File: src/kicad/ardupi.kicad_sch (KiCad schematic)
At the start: 58 parts, among them J1 RPI-4B-Header, J10 Conn_01x04, J11 TSW-108-08-L-T-RA, J2 Conn_01x10, J3 Conn_01x05, J4 Conn_01x04, J6 Conn_01x05, J7 Conn_01x06, J8 Conn_01x04, J9 Conn_01x02, U1 CAT24C256, U2 ULN2803ADW, U3 PCA9685PW, U4 ADS1115IRUGR, U5 MPU-9250, U6 BMP280

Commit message: version bump
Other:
- title: (none) -> ArduPi
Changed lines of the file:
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@@
   (paper "A3")
   (title_block
-    (date "15 nov 2012")
+    (title "ArduPi")
+    (date "2022-06-05")
+    (rev "0.1.4")
+    (comment 1 "Author: Muhammad Hefny")
+    (comment 2 "Author: Shaun Lloyd")
   )
   (junction (at 325.12 66.04) (diameter 0) (color 0 0 0 0)

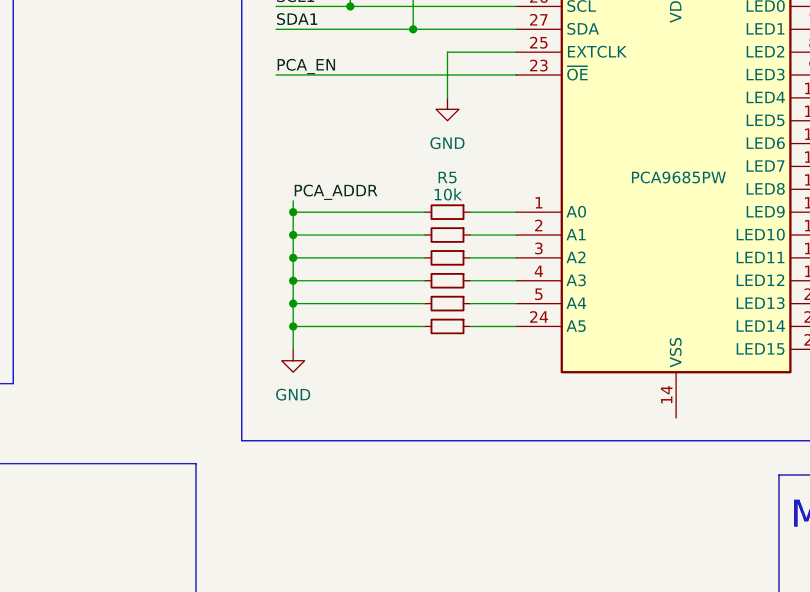
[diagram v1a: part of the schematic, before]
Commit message: elec: PCA9685 jumpers
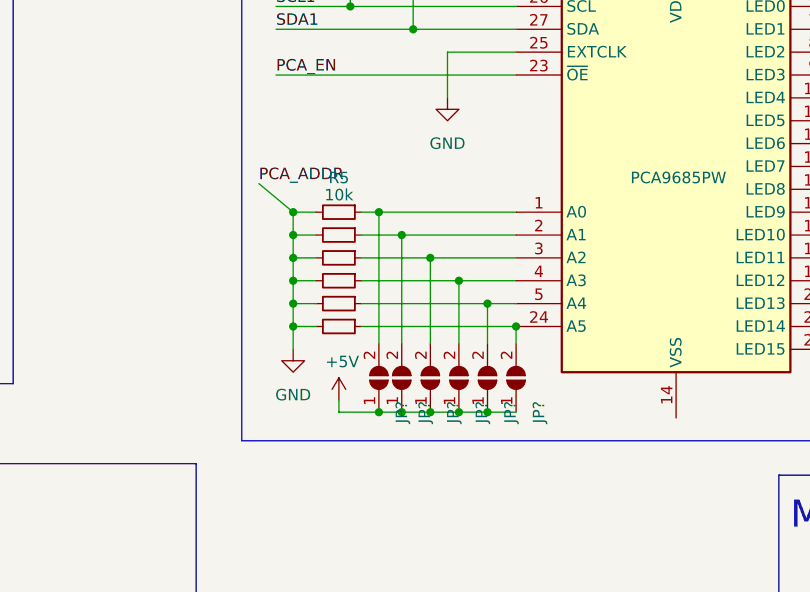
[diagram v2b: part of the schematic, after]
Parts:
- added JP? (x6): ID_WP, symbol Jumper:SolderJumper_2_Open
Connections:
- net +5V: now also JP?.1 (A), JP?.1 (A), JP?.1 (A), JP?.1 (A), JP?.1 (A), JP?.1 (A)
- net at R7.1, U3.3 (A2): now also JP?.2 (B)
- net at R6.1, U3.2 (A1): now also JP?.2 (B)
- net at R5.1, U3.1 (A0): now also JP?.2 (B)
- net at R10.1, U3.24 (A5): now also JP?.2 (B)
- net at R8.1, U3.4 (A3): now also JP?.2 (B)
- net at R9.1, U3.5 (A4): now also JP?.2 (B)
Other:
- moved on the sheet: R5
